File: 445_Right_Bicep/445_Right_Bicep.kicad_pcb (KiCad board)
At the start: 2 copper layers, 60.1 x 48.6 mm, 0 parts

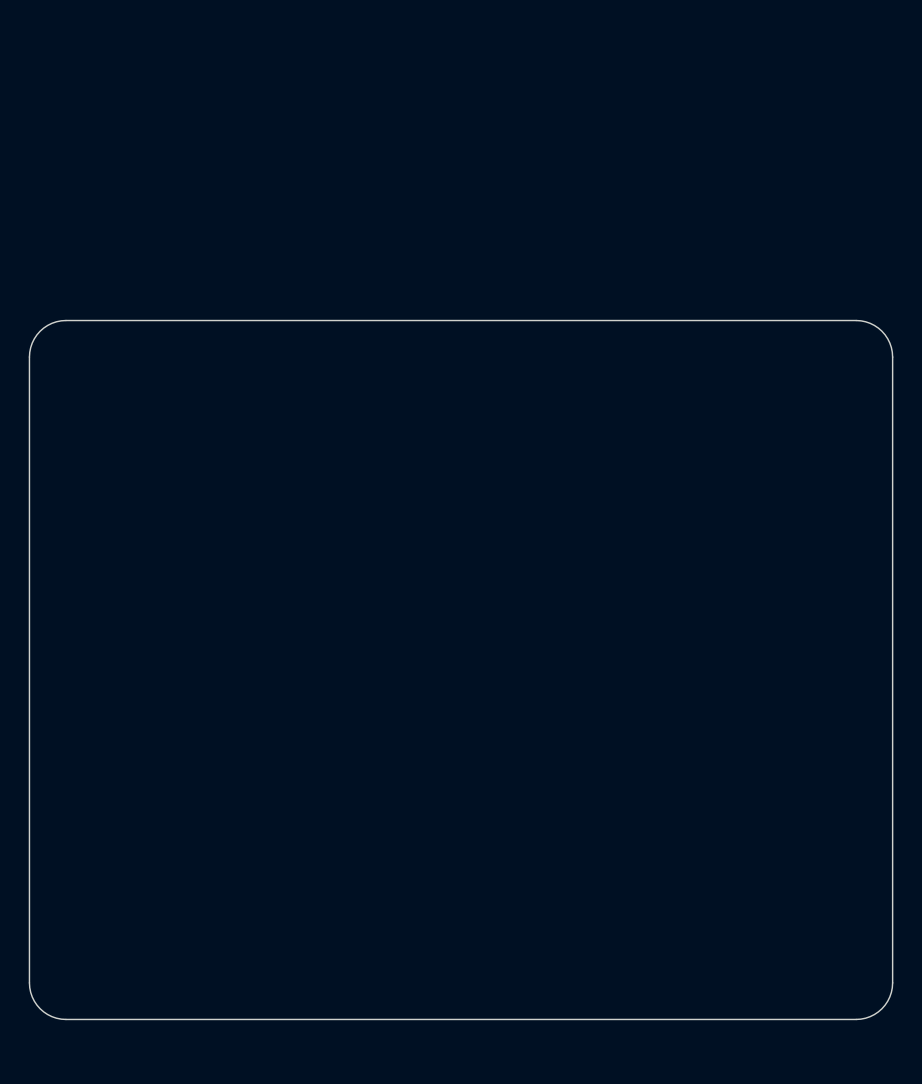
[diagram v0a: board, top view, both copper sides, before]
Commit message: Layout First Draft
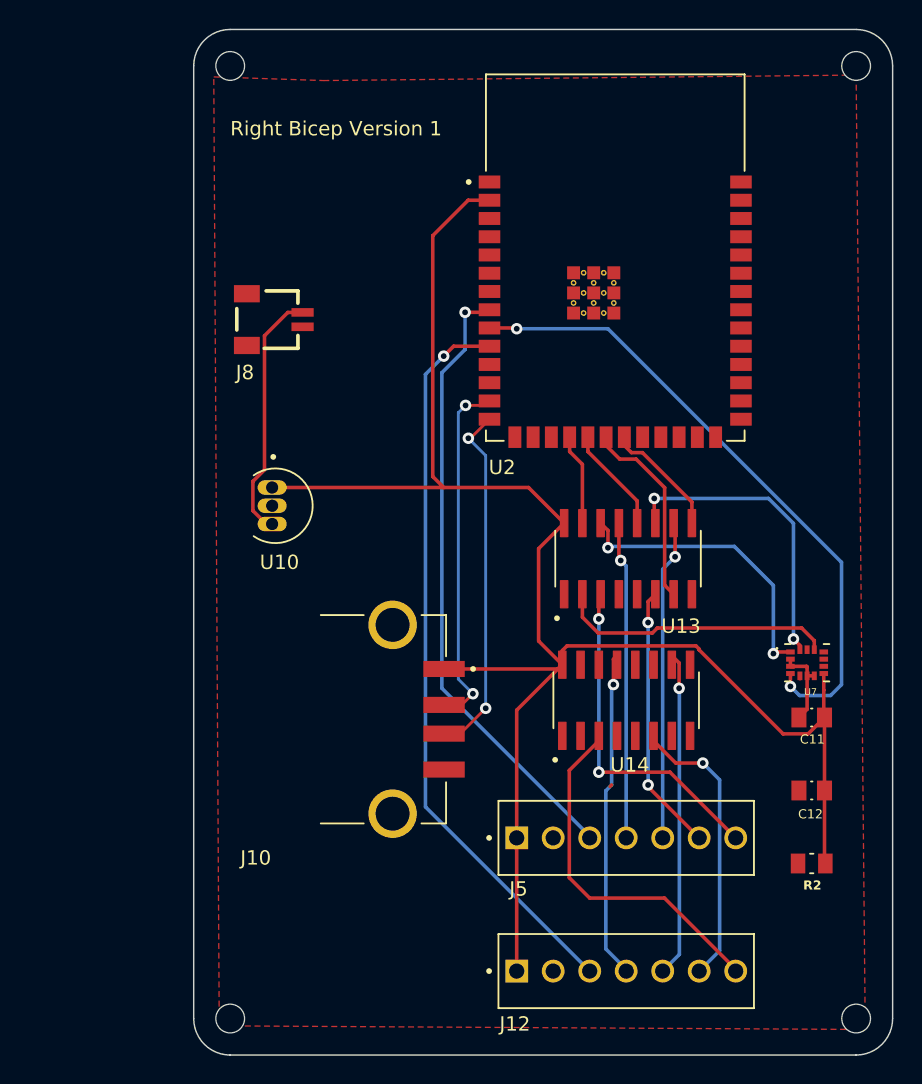
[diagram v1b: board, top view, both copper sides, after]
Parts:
- added C11: 100nF, CL21F104ZAANNNC:CAPC2012X135N, F.Cu at (164.9, 97.0)
- added C12: 100nF, CL21F104ZAANNNC:CAPC2012X135N, F.Cu at (164.9, 102.1)
- added H1: MountingHole, MountingHole:MountingHole_2mm, F.Cu at (124.5, 51.7)
- added H2: MountingHole, MountingHole:MountingHole_2mm, F.Cu at (168.0, 51.7)
- added H3: MountingHole, MountingHole:MountingHole_2mm, F.Cu at (124.5, 118.0)
- added H4: MountingHole, MountingHole:MountingHole_2mm, F.Cu at (168.0, 118.0)
- added J10: 87583-2010RPLF, 87583-2010RPLF:AMPHENOL_87583-2010RPLF, F.Cu at (135.8, 97.2)
- added J12: 69167-107HLF, 69167-107HLF:AMPHENOL_69167-107HLF, F.Cu at (152.0, 114.7)
- added J5: 69167-107HLF, 69167-107HLF:AMPHENOL_69167-107HLF, F.Cu at (152.0, 105.4)
- added J8: SM02B-SRSS-TB_LF__SN_, SM02B-SRSS-TB_LF__SN_:SM02B-SRSS-TB_LF__SN_, F.Cu at (127.5, 69.3)
- added R2: 10k, RMCF0805JG10K0:RESC2012X65N, F.Cu at (164.9, 107.2)
- added U10: LP2950CZ-3.3_LFT3, LP2950CZ-3.3_LFT3:TO92127P521H735-3, F.Cu at (128.2, 82.3)
- added U13: TS3A5018D, TS3A5018D:SOIC127P600X175-16N, F.Cu at (152.1, 86.0)
- added U14: TS3A5018D, TS3A5018D:SOIC127P600X175-16N, F.Cu at (152.0, 95.8)
- added U2: ESP32-S3-WROOM-1-N16R8, ESP32-S3-WROOM-1-N16R8:XCVR_ESP32-S3-WROOM-1-N16R8, F.Cu at (151.3, 65.0)
- added U7: LSM6DSMTR, LSM6DSMTR (1):PQFN50P300X250X86-14N, F.Cu at (164.6, 93.2)
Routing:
- net +3.3V: track 0.00 -> 123.1 mm
- net INT1_3: track 0.00 -> 51.7 mm, vias 0 -> 1
- net INT1_2: track 0.00 -> 44.8 mm, vias 0 -> 2
- net INT1_1: track 0.00 -> 43.3 mm, vias 0 -> 1
- net SENSOR_3: track 0.00 -> 25.7 mm
- net D+: track 0.00 -> 24.9 mm, vias 0 -> 2
- net D-: track 0.00 -> 24.8 mm, vias 0 -> 2
- net SENSOR_1: track 0.00 -> 23.9 mm, vias 0 -> 2
- net MISO_3: track 0.00 -> 22.9 mm, vias 0 -> 1
- net MOSI_3: track 0.00 -> 22.7 mm, vias 0 -> 1
- net MOSI_1: track 0.00 -> 22.3 mm, vias 0 -> 1
- net MISO_1: track 0.00 -> 22.1 mm, vias 0 -> 1
- net MOSI_2: track 0.00 -> 21.1 mm, vias 0 -> 2
- net CLK3: track 0.00 -> 20.6 mm, vias 0 -> 1
- net MISO_2: track 0.00 -> 20.4 mm, vias 0 -> 2
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- added copper zone on F.Cu, net (none)
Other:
- board size 60.1 x 48.6 mm -> 48.6 x 71.4 mm
- board text added: "Right Bicep Version 1"
